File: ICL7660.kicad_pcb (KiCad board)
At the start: 2 copper layers, 38.1 x 31.8 mm, 14 parts, among them J1 Vin, J2 GND, J3 Vout, J4 GND, J5 -Vout, U1 ICL7660

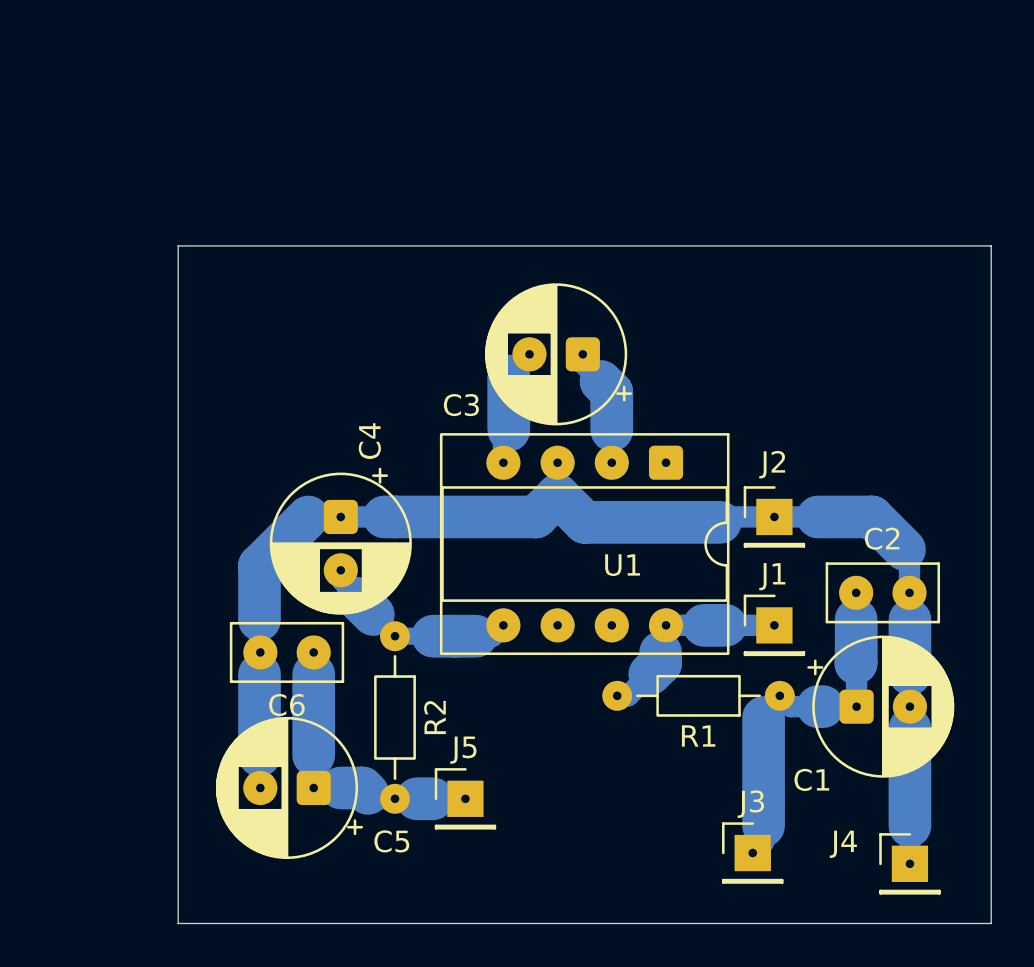
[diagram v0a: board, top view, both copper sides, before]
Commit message: 配置を修正
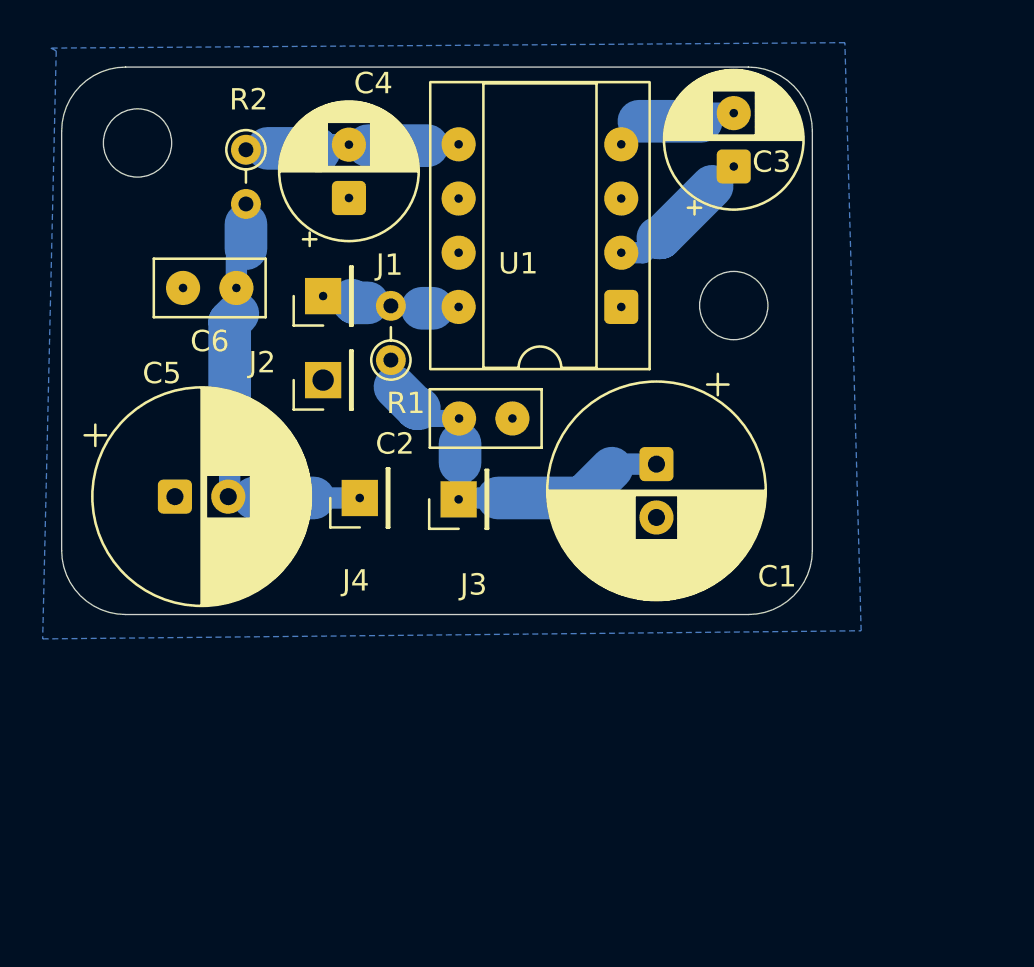
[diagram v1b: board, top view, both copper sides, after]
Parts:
- removed the J4 at (154.9, 95.0)
- added H1: MountingHole, MountingHole:MountingHole_3.2mm_M3, F.Cu at (118.7, 61.2)
- added H2: MountingHole, MountingHole:MountingHole_3.2mm_M3, F.Cu at (146.7, 68.8)
- C1, C5: footprint Capacitor_THT:CP_Radial_D6.3mm_P2.50mm -> Capacitor_THT:CP_Radial_D10.0mm_P2.50mm
- R1, R2: footprint Resistor_THT:R_Axial_DIN0204_L3.6mm_D1.6mm_P7.62mm_Horizontal -> Resistor_THT:R_Axial_DIN0204_L3.6mm_D1.6mm_P2.54mm_Vertical
- moved J1 26.2 mm to (127.4, 68.4), turned to 90 degrees
- moved R1 24.1 mm to (130.6, 71.4), turned to 90 degrees
- moved R2 23.8 mm to (123.8, 61.5)
- moved J2 22.1 mm to (127.4, 72.3), turned to 90 degrees
- moved J3 21.6 mm to (133.8, 77.9), turned to 90 degrees
- moved C2 20.3 mm to (133.8, 74.1)
- moved C6 17.5 mm to (123.4, 68.0)
- moved C5 15.1 mm to (120.5, 77.8), turned to 0 degrees
- moved C4 15.0 mm to (128.7, 63.8), turned to 90 degrees
- moved J4 14.9 mm to (129.2, 77.9), turned to 90 degrees
- moved C1 14.7 mm to (143.1, 76.3), turned to -90 degrees
- moved C3 11.3 mm to (146.7, 62.3), turned to 90 degrees
- moved U1 7.60 mm to (141.4, 68.9), turned to 180 degrees
- renumbered J5 to J4
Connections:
- C5 pad 1: Net-(J5-Pin_1) -> GND
- C5 pad 2: GND -> Net-(J4-Pin_1)
- C6 pad 1: Net-(J5-Pin_1) -> Net-(J4-Pin_1)
- J4 pad 1: Net-(J5-Pin_1) -> Net-(J4-Pin_1)
- R2 pad 2: Net-(J5-Pin_1) -> Net-(J4-Pin_1)
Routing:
- net GND: track 68.1 -> 0.00 mm
- net Net-(J4-Pin_1): track 0.00 -> 20.3 mm
- net Net-(J5-Pin_1): track 14.4 -> 0.00 mm
- net Net-(J1-Pin_1): track 9.63 -> 5.10 mm
- net Net-(J3-Pin_1): track 22.4 -> 19.1 mm
- net Net-(U1-CAP+): track 5.64 -> 7.04 mm
- net Net-(U1-VOUT): track 9.43 -> 10.2 mm
- added copper zone on B.Cu, net GND
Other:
- board size 38.1 x 31.8 mm -> 35.2 x 25.7 mm
